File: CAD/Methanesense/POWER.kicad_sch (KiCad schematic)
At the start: 27 parts, among them J1 USB_C_Receptacle_USB2.0_14P, SW3 KMR223NGLFG, U3 nPM1300-QEXX, U4 AP7331-20WG-7, U7 FT230XQ

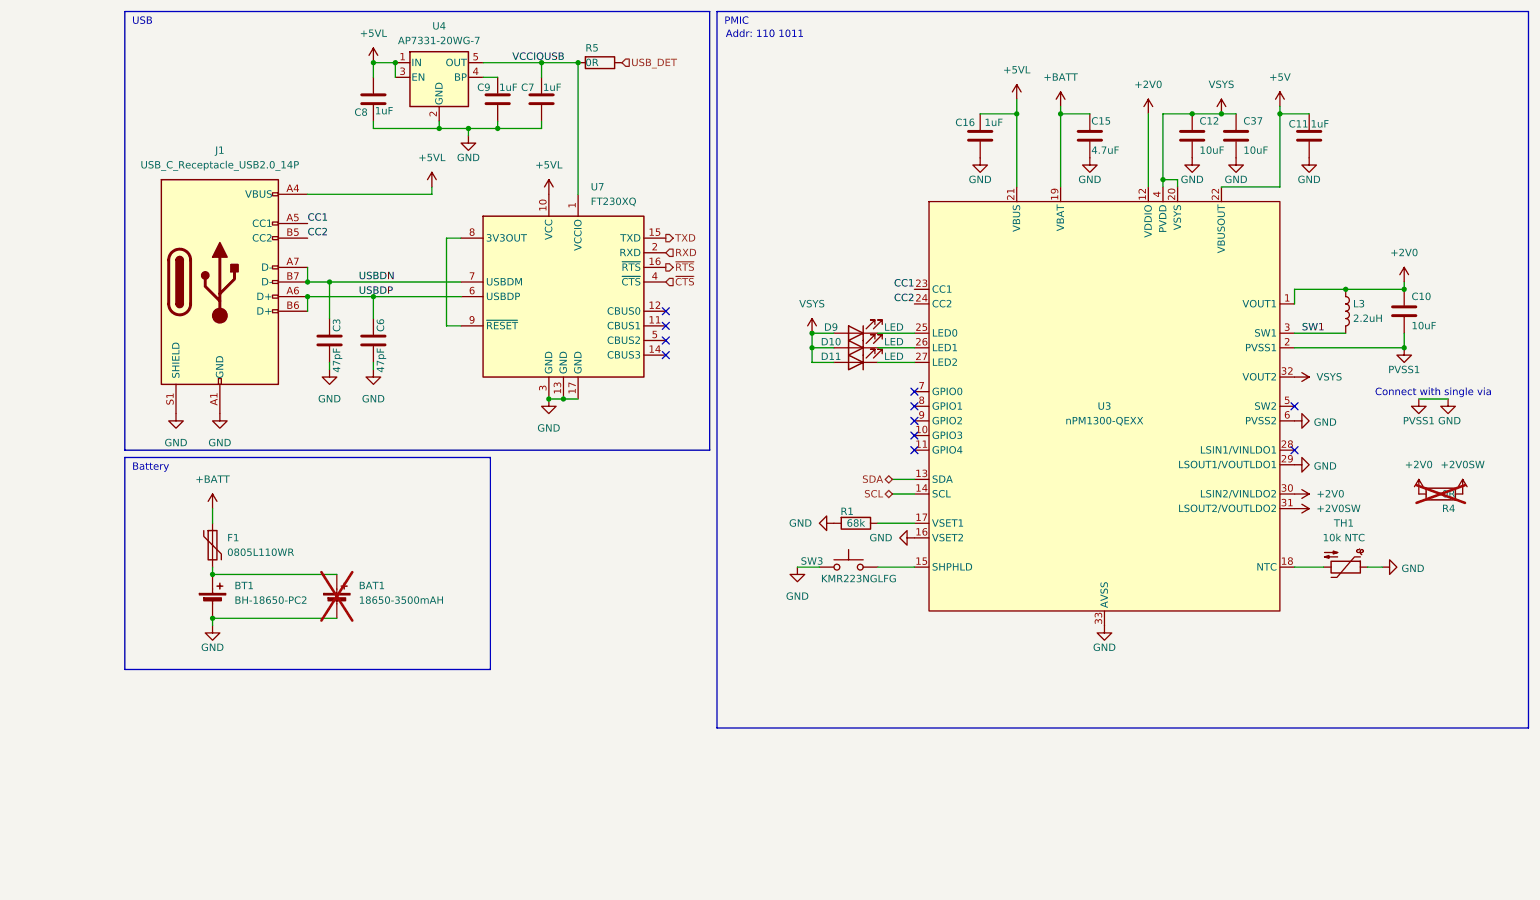
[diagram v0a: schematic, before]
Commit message: rev 1.2
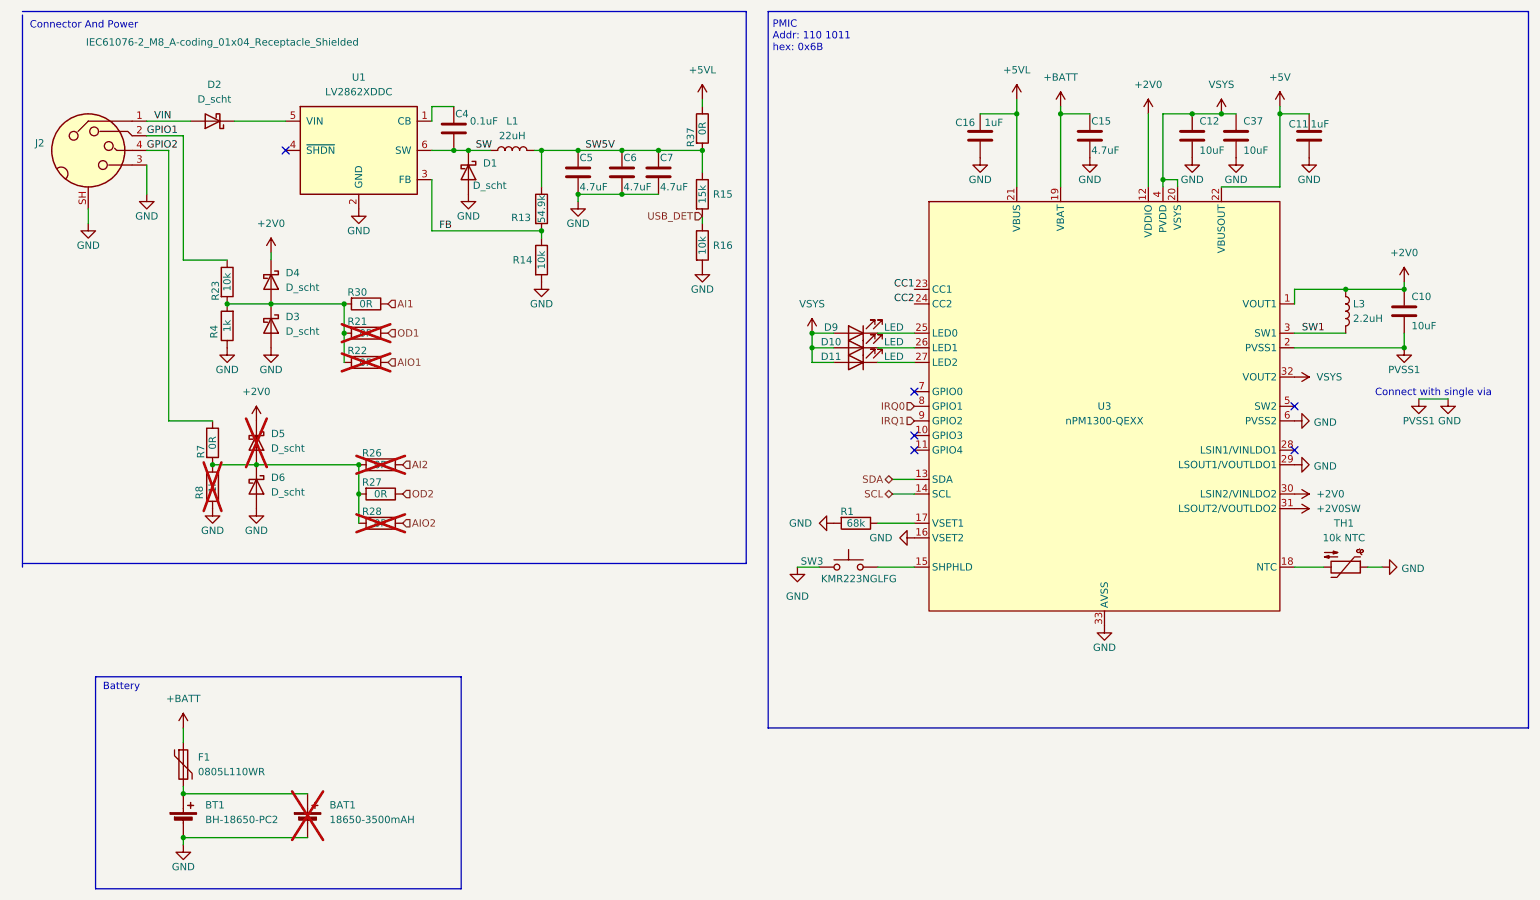
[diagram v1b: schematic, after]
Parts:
- removed C3, C6: 47pF, Capacitor_SMD:C_0603_1608Metric, symbol Library:C
- removed C7, C8, C9: 1uF, Capacitor_SMD:C_0603_1608Metric, symbol Library:C
- removed J1: USB_C_Receptacle_USB2.0_14P, Methanesense:USB_C_Receptacle_HCTL_HC-TYPE-C-16P-01A, symbol Connector:USB_C_Receptacle_USB2.0_14P
- removed R5: 0R, Resistor_SMD:R_0603_1608Metric, symbol Library:R
- removed U4: AP7331-20WG-7, Package_TO_SOT_SMD:SOT-23-5, symbol Regulator_Linear:AP131-20
- removed U7: FT230XQ, Methanesense:QFN-16-1EP_4x4mm_P0.65mm_EP2.1x2.1mm, symbol Interface_USB:FT230XQ
- added C4: 0.1uF, Capacitor_SMD:C_0603_1608Metric, symbol Device:C
- added C5, C6, C7: 4.7uF, Capacitor_SMD:C_0603_1608Metric, symbol Device:C
- added D1, D2: D_scht, Diode_SMD:D_MicroSMP_AK, symbol Device:D_Schottky
- added D3, D4, D5, D6: D_scht, Diode_SMD:D_0603_1608Metric, symbol Device:D_Schottky
- added J2: IEC61076-2_M8_A-coding_01x04_Receptacle_Shielded, Methanesense:STEWART_SS-12800-004_M8_04_Socket_Right_Angle, symbol Connector:IEC61076-2_M8_A-coding_01x04_Receptacle_Shielded
- added L1: 22uH, Methanesense:L_Abracon_AMDLA4020S, symbol Device:L
- added R13: 54.9k, Resistor_SMD:R_0603_1608Metric, symbol Library:R
- added R14, R16, R23: 10k, Resistor_SMD:R_0603_1608Metric, symbol Library:R
- added R15: 15k, Resistor_SMD:R_0603_1608Metric, symbol Library:R
- added R21, R22, R26, R27, R28, R30, R37, R7: 0R, Resistor_SMD:R_0603_1608Metric, symbol Library:R
- added R8: 1k, Resistor_SMD:R_0603_1608Metric, symbol Library:R
- added U1: LV2862XDDC, Package_TO_SOT_SMD:SOT-23-6, symbol Regulator_Switching:LV2862XDDC
- R4: value 0R -> 1k; now fitted
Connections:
- net +2V0: now also D4.1 (K), D5.1 (K); no longer R4.1
- net +2V0SW: no longer R4.2
- net +5VL: now also R37.1
- net GND: now also R4.1, C5.2, C6.2, C7.2, D1.2 (A), D3.2 (A), D6.2 (A), J2.3, J2.SH, R14.2, R16.2, R8.1, U1.2 (GND)
- net USB_DET: now also R15.2, R16.1
- net IRQ0: now reaches U3.8 (GPIO1)
- net IRQ1: now reaches U3.9 (GPIO2)
- new net: C4.1, U1.1 (CB)
- new net: D2.1 (K), U1.5 (VIN)
- new net: D5.2 (A), D6.1 (K), R26.2, R27.2, R28.2, R7.2, R8.2
- new net: D3.1 (K), D4.2 (A), R21.2, R22.2, R23.2, R30.2, R4.2
- new net AI1: R30.1
- new net AI2: R26.1
- new net AIO1: R22.1
- new net AIO2: R28.1
- new net FB: R13.2, R14.1, U1.3 (FB)
- new net GPIO1: J2.2, R23.1
- new net GPIO2: J2.4, R7.1
- new net OD1: R21.1
- new net OD2: R27.1
- new net SW: C4.2, D1.1 (K), L1.1, U1.6 (SW)
- new net SW5V: C5.1, C6.1, C7.1, L1.2, R13.1, R15.1, R37.2
- new net VIN: D2.2 (A), J2.1
- no-connect marks 11 -> 6
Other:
- note added: "Addr: 110 1011 hex: 0x6B"
- note added: "Connector And Power"
- note removed: "Addr: 110 1011"
- note removed: "USB"
- moved on the sheet: BAT1, BT1, F1
